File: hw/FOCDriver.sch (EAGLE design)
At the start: 111 parts, among them Q1 BC817, Q2 BC817, Q3 BC817, Q4 BC817, Q5 BC817, Q6 BC817, Q7 IRFR5305, U10 SN74LVC2G17, U11 SN74LVC2G17, U12 SN74LVC2G17, U2 BA7805FP, U5 LM358N, U6 LM358N, U7 AO4606, U8 AO4606, U9 AO4606

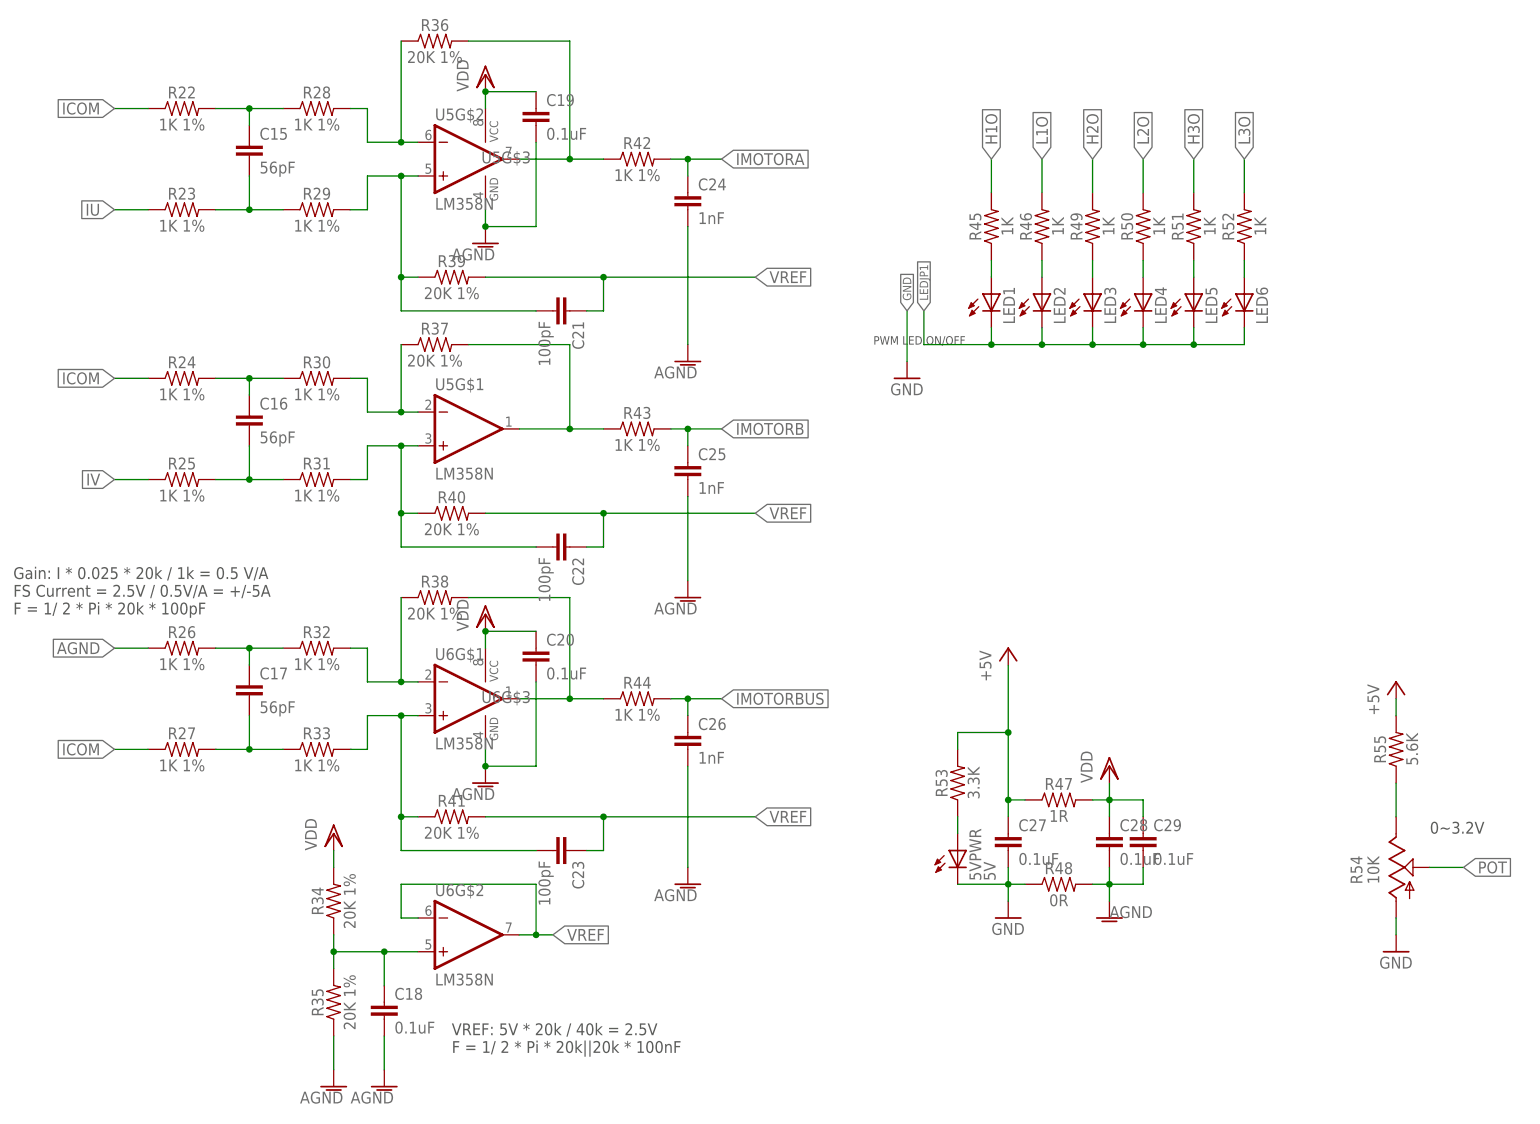
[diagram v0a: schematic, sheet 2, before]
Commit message: layout
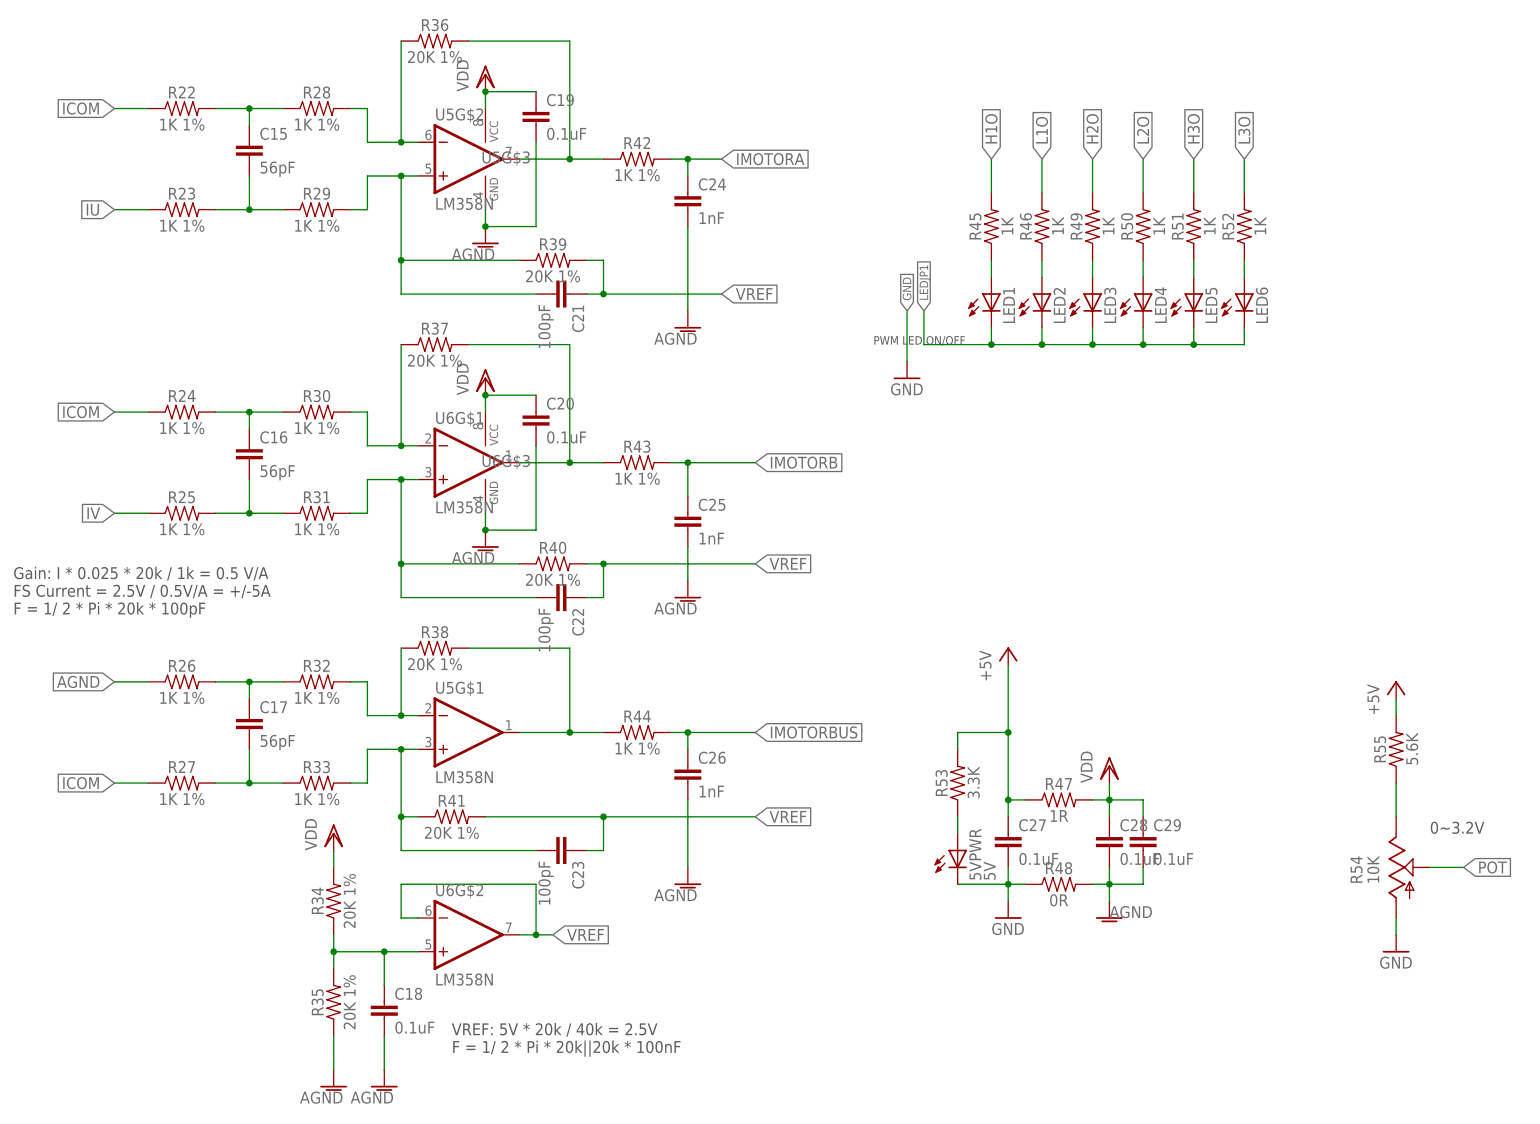
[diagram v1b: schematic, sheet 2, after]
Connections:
- new net VDD: C19.1, U5G$3.VCC
- net AVDD: no longer C19.1, U5G$3.VCC
- net N$19: now also U6G$1.-IN; no longer U5G$1.-IN
- net N$20: now also U6G$1.+IN; no longer U5G$1.+IN
- net N$21: now also U6G$1.OUT; no longer U5G$1.OUT
- net N$24: now also U5G$1.-IN; no longer U6G$1.-IN
- net N$25: now also U5G$1.+IN; no longer U6G$1.+IN
- net N$26: now also U5G$1.OUT; no longer U6G$1.OUT
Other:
- moved on the sheet: C16, C17, C20, C21, C22, C25, C26, R24, R25, R26, R27, R30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
